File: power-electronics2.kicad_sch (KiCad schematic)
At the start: 8 parts, among them IC1 UC2843BD1, IC2 ZTL431AFFTA, J1 Vin, Q1 STP16NF06, U1 4N35

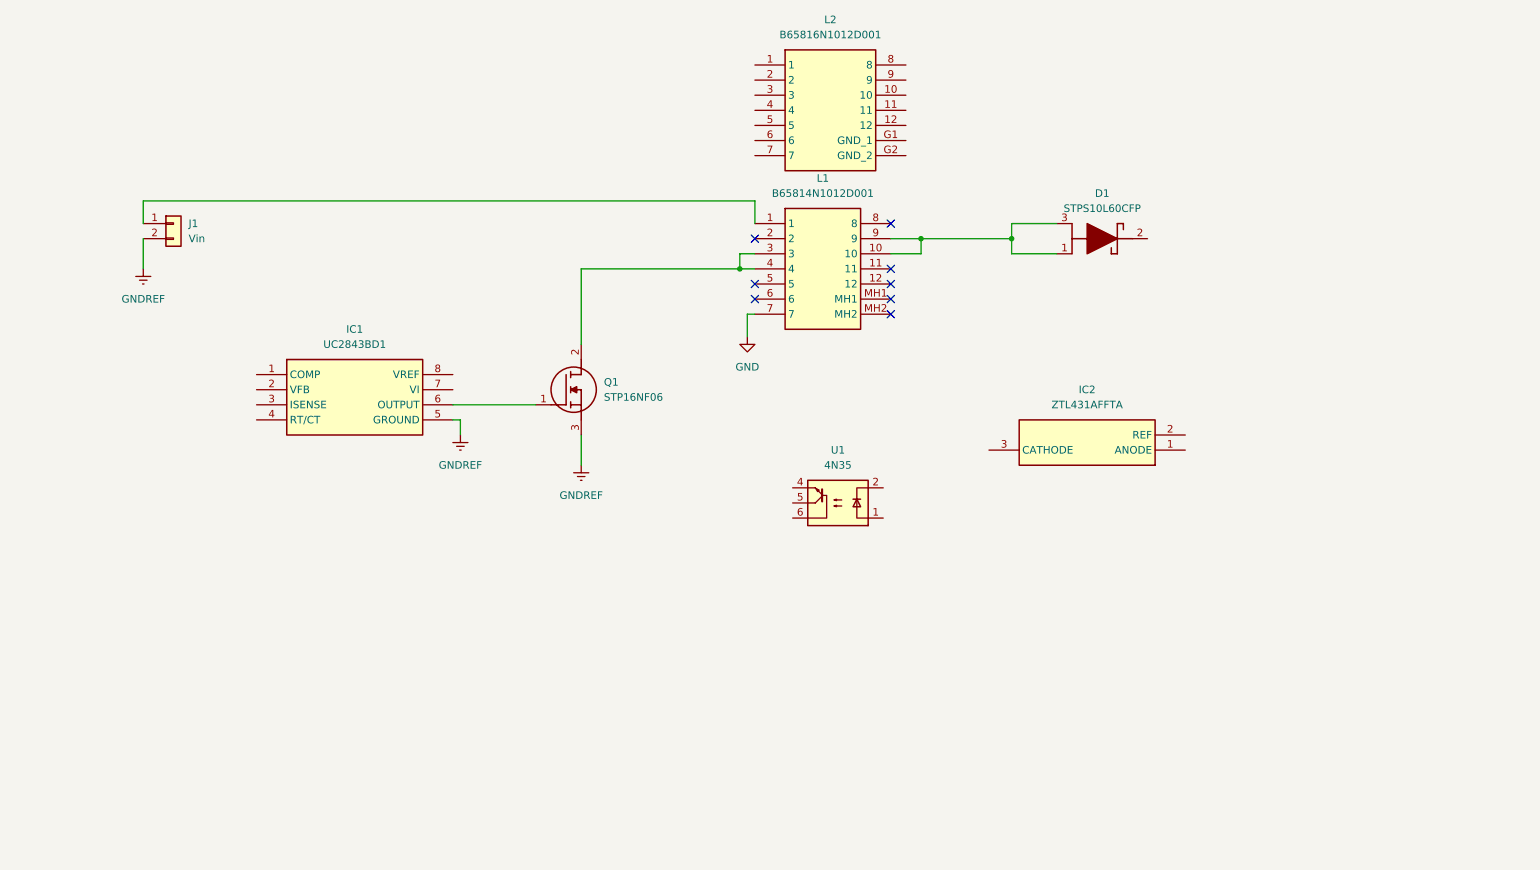
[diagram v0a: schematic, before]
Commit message: finish pcb
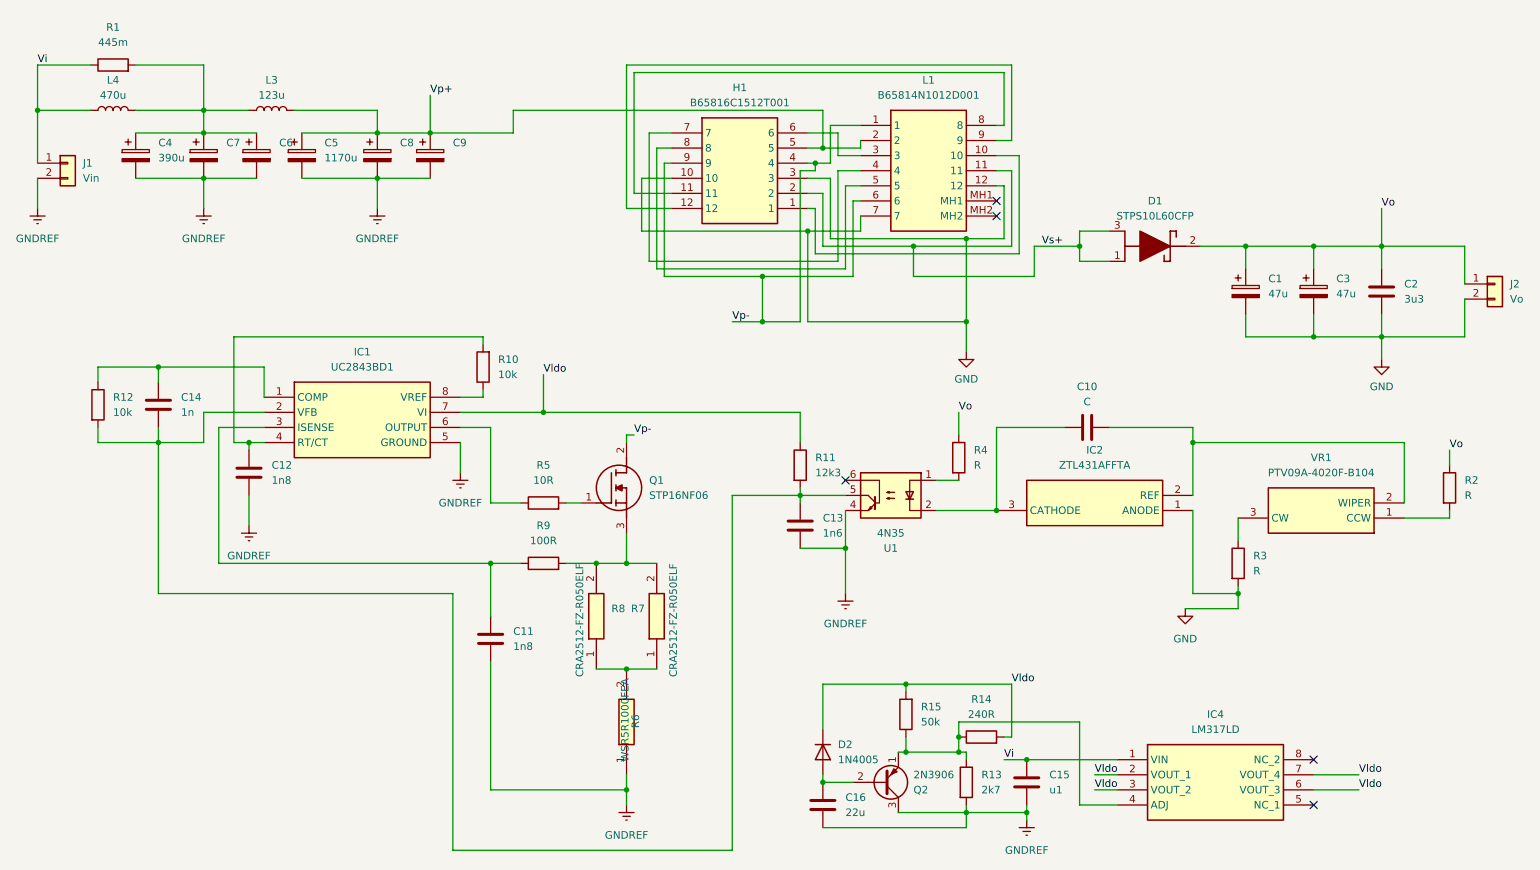
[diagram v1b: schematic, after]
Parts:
- removed L2: B65816N1012D001, Samacsys:B65816N1012D001, symbol Samacsys:B65816N1012D001
- added C1, C3: 47u, Capacitor_THT:CP_Radial_D10.0mm_P5.00mm, symbol Device:C_Polarized
- added C10: C, Capacitor_SMD:C_0805_2012Metric_Pad1.18x1.45mm_HandSolder, symbol Device:C
- added C11, C12: 1n8, Capacitor_SMD:C_0805_2012Metric_Pad1.18x1.45mm_HandSolder, symbol Device:C
- added C13: 1n6, Capacitor_SMD:C_0805_2012Metric_Pad1.18x1.45mm_HandSolder, symbol Device:C
- added C14: 1n, Capacitor_SMD:C_0805_2012Metric_Pad1.18x1.45mm_HandSolder, symbol Device:C
- added C15: u1, Capacitor_SMD:C_0805_2012Metric_Pad1.18x1.45mm_HandSolder, symbol Device:C
- added C16: 22u, Capacitor_SMD:C_0805_2012Metric_Pad1.18x1.45mm_HandSolder, symbol Device:C
- added C2: 3u3, Capacitor_THT:C_Axial_L12.0mm_D7.5mm_P15.00mm_Horizontal, symbol Device:C
- added C4: 390u, Capacitor_THT:CP_Radial_D10.0mm_P5.00mm, symbol Device:C_Polarized
- added C5: 1170u, Capacitor_THT:CP_Radial_D16.0mm_P7.50mm, symbol Device:C_Polarized
- added C6, C7, C8, C9: C, Capacitor_THT:CP_Radial_D10.0mm_P5.00mm, symbol Device:C_Polarized
- added D2: 1N4005, Diode_THT:D_DO-41_SOD81_P10.16mm_Horizontal, symbol Diode:1N4005
- added H1: B65816C1512T001, Samacsys:B65816C1512T001, symbol Samacsys:B65816C1512T001
- added IC4: LM317LD, Samacsys:SOIC127P600X175-8N, symbol Samacsys:LM317LD
- added J2: Vo, Connector_Wire:SolderWire-1.5sqmm_1x02_P6mm_D1.7mm_OD3mm, symbol Connector_Generic:Conn_01x02
- added L3: 123u, Inductor_THT:L_Axial_L29.9mm_D14.0mm_P38.00mm_Horizontal_Vishay_IHA-105, symbol Device:L
- added L4: 470u, Inductor_THT:L_Axial_L29.9mm_D14.0mm_P38.00mm_Horizontal_Vishay_IHA-105, symbol Device:L
- added Q2: 2N3906, Package_TO_SOT_THT:TO-92_Inline, symbol Transistor_BJT:2N3906
- added R1: 445m, Resistor_SMD:R_0805_2012Metric_Pad1.20x1.40mm_HandSolder, symbol Device:R
- added R10, R12: 10k, Resistor_SMD:R_0805_2012Metric_Pad1.20x1.40mm_HandSolder, symbol Device:R
- added R11: 12k3, Resistor_SMD:R_0805_2012Metric_Pad1.20x1.40mm_HandSolder, symbol Device:R
- added R13: 2k7, Resistor_SMD:R_0805_2012Metric_Pad1.20x1.40mm_HandSolder, symbol Device:R
- added R14: 240R, Resistor_SMD:R_0805_2012Metric_Pad1.20x1.40mm_HandSolder, symbol Device:R
- added R15: 50k, Resistor_SMD:R_0805_2012Metric_Pad1.20x1.40mm_HandSolder, symbol Device:R
- added R2, R3, R4: R, Resistor_SMD:R_0805_2012Metric_Pad1.20x1.40mm_HandSolder, symbol Device:R
- added R5: 10R, Resistor_SMD:R_0805_2012Metric_Pad1.20x1.40mm_HandSolder, symbol Device:R
- added R6: WSR5R1000FEA, Samacsys:RESM11670X254N, symbol Samacsys:WSR5R1000FEA
- added R7, R8: CRA2512-FZ-R050ELF, Samacsys:RESC6434X90N, symbol Samacsys:CRA2512-FZ-R050ELF
- added R9: 100R, Resistor_SMD:R_0805_2012Metric_Pad1.20x1.40mm_HandSolder, symbol Device:R
- added VR1: PTV09A-4020F-B104, Samacsys:PTV09A4020FB103, symbol Samacsys:PTV09A-4020F-B104
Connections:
- net GND: now also IC2.1 (ANODE), L1.12, C1.2, C2.2, C3.2, H1.10, H1.3, J2.2 (Pin_2), R3.2
- net GNDREF: now also U1.4, C11.2, C12.2, C13.2, C15.2, C16.2, C4.2, C5.2, C6.2, C7.2, C8.2, C9.2, Q2.3 (C), R13.2, R6.1; no longer Q1.3 (S)
- net Vi: now reaches J1.1 (Pin_1)
- net Vi: now also C15.1, IC4.1 (VIN), L4.1, R1.1; no longer L1.1
- net Vs+: now reaches D1.1 (A1), D1.3 (A2)
- net Vs+: now also L1.11, H1.2; no longer L1.10, L1.9
- net Vp+: now reaches L1.2
- net Vp+: now also C5.1, C8.1, C9.1, H1.5, L3.2
- net at L1.5: now also H1.8
- net Vp-: now reaches L1.6
- net Vp-: now also L1.1, Q1.2 (D), H1.4, H1.9
- net at L1.8: now also H1.11
- net at Q1.1 (G): now also R5.2; no longer IC1.6 (OUTPUT)
- net at IC2.2 (REF): now also C10.2, VR1.2 (WIPER)
- net at IC2.3 (CATHODE): now also U1.2, C10.1
- net at IC1.1 (COMP): now also C14.1, R12.1
- net at IC1.2 (VFB): now also U1.5, C13.1, C14.2, R11.2, R12.2
- net at IC1.3 (ISENSE): now also C11.1, R9.1
- net at IC1.4 (RT/CT): now also C12.1, R10.2
- net Vldo: now reaches IC1.7 (VI)
- net Vldo: now also D2.1 (K), IC4.2 (VOUT_1), IC4.3 (VOUT_2), IC4.6 (VOUT_3), IC4.7 (VOUT_4), R11.1, R14.2, R15.2
- net at IC1.8 (VREF): now also R10.1
- net Vo: now reaches D1.2 (K)
- net Vo: now also C1.1, C2.1, C3.1, J2.1 (Pin_1), R2.1, R4.1
- net at U1.1: now also R4.2
- new net: IC4.4 (ADJ), Q2.1 (E), R13.1, R14.1, R15.1
- new net: C4.1, C6.1, C7.1, L3.1, L4.2, R1.2
- new net: Q1.3 (S), R7.2, R8.2, R9.2
- new net: R6.2, R7.1, R8.1
- new net: C16.1, D2.2 (A), Q2.2 (B)
- new net: R2.2, VR1.1 (CCW)
- new net: R3.1, VR1.3 (CW)
- new net: IC1.6 (OUTPUT), R5.1
- new net: H1.1, L1.10
- new net: H1.12, L1.9
- new net: H1.6, L1.3
- new net: H1.7, L1.4
- no-connect marks 8 -> 5
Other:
- moved on the sheet: D1, IC1, IC2, J1, Q1, U1
